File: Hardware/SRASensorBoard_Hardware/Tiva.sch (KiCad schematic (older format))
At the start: 7 parts, among them U3 TM4C129E_Launchpad

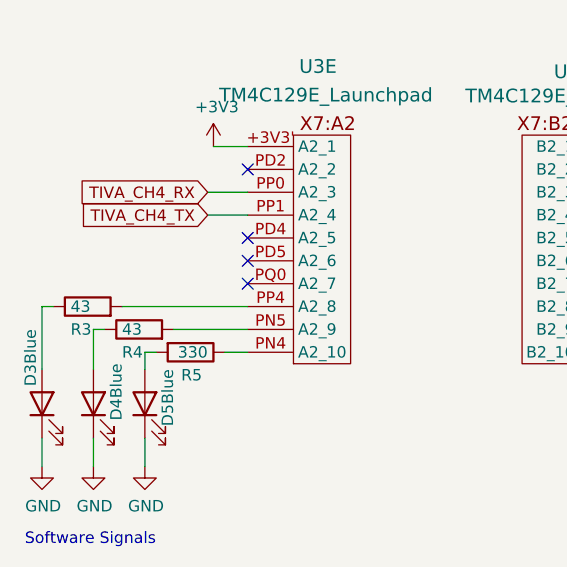
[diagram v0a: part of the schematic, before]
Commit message: rev 2 changes
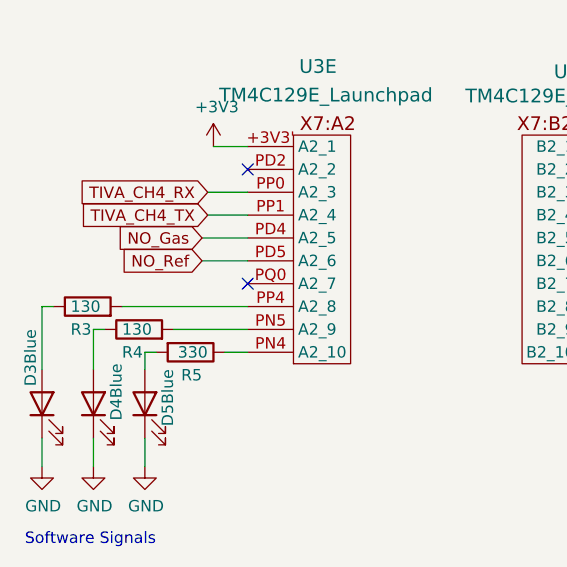
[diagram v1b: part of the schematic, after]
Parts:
- R3, R4: value 43 -> 130
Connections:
- net NO_Gas: now reaches U3.PD4 (A2_5)
- net NO_Ref: now reaches U3.PD5 (A2_6)
- no-connect marks 52 -> 50
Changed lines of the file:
@@
 Wire Wire Line
 	2000 3400 2175 3400
-Text GLabel 1850 2275 0    50   Output ~ 0
-NO2_SCL
-Text GLabel 1850 2375 0    50   Output ~ 0
-NO2_SDA
-Wire Wire Line
-	2125 2275 1850 2275
-Wire Wire Line
-	2125 2375 1850 2375
 Text GLabel 4000 3500 2    50   Input ~ 0
 TIVA_NH3_A
@@
 NoConn ~ 2125 2075
 NoConn ~ 2175 3200
-NoConn ~ 2175 3500
-NoConn ~ 2175 3600
 NoConn ~ 2175 3700
 NoConn ~ 3825 4000
@@
 NoConn ~ 6975 3825
 NoConn ~ 6975 3925
-$Comp
-L Device:LED D4
-U 1 1 6165658F
-P 1500 4225
-F 0 "D4" H 1475 4125 50  0000 C CNN
-F 1 "Blue" H 1600 4125 50  0000 C CNN
-F 2 "LED_SMD:LED_0603_1608Metric_Pad1.05x0.95mm_HandSolder" H 1500 4225 50  0001 C CNN
-F 3 "~" H 1500 4225 50  0001 C CNN
-	1    1500 4225
-	0    -1   -1   0
-$EndComp
-Wire Wire Line
-	2175 3800 1625 3800
-Wire Wire Line
-	1850 3900 2175 3900
-Wire Wire Line
-	2075 4000 2175 4000
-Wire Wire Line
-	1775 4000 1725 4000
-Wire Wire Line
-	1725 4000 1725 4075
-$Comp
-L Device:R R4
-U 1 1 6165C9F3
-P 1700 3900
-F 0 "R4" V 1600 3975 50  0000 R CNN
-F 1 "43" V 1700 3975 50  0000 R CNN
-F 2 "Resistor_SMD:R_0603_1608Metric_Pad1.05x0.95mm_HandSolder" V 1630 3900 50  0001 C CNN
-F 3 "~" H 1700 3900 50  0001 C CNN
-	1    1700 3900
-	0    -1   -1   0
-$EndComp
-$Comp
-L Device:R R3
-U 1 1 6165CD26
-P 1475 3800
-F 0 "R3" V 1375 3875 50  0000 R CNN
-F 1 "43" V 1475 3875 50  0000 R CNN
-F 2 "Resistor_SMD:R_0603_1608Metric_Pad1.05x0.95mm_HandSolder" V 1405 3800 50  0001 C CNN
-F 3 "~" H 1475 3800 50  0001 C CNN
-	1    1475 3800
-	0    -1   -1   0
-$EndComp
-$Comp
-L Device:LED D3
-U 1 1 616555A2
-P 1275 4225
-F 0 "D3" H 1400 4275 50  0000 C CNN
-F 1 "Blue" H 1525 4275 50  0000 C CNN
-F 2 "LED_SMD:LED_0603_1608Metric_Pad1.05x0.95mm_HandSolder" H 1275 4225 50  0001 C CNN
-F 3 "~" H 1275 4225 50  0001 C CNN
-	1    1275 4225
-	0    -1   -1   0
-$EndComp
-Wire Wire Line
-	1550 3900 1500 3900
-Wire Wire Line
-	1500 3900 1500 4075
-Wire Wire Line
-	1325 3800 1275 3800
-Wire Wire Line
-	1275 3800 1275 4075
-$Comp
-L power:GND #PWR0119
-U 1 1 61666E76
-P 1500 4500
-F 0 "#PWR0119" H 1500 4250 50  0001 C CNN
-F 1 "GND" H 1505 4327 50  0000 C CNN
-F 2 "" H 1500 4500 50  0001 C CNN
-F 3 "" H 1500 4500 50  0001 C CNN
-	1    1500 4500
-	1    0    0    -1
-$EndComp
-$Comp
-L power:GND #PWR0120
-U 1 1 6166AD67
-P 1725 4500
-F 0 "#PWR0120" H 1725 4250 50  0001 C CNN
-F 1 "GND" H 1730 4327 50  0000 C CNN
-F 2 "" H 1725 4500 50  0001 C CNN
-F 3 "" H 1725 4500 50  0001 C CNN
-	1    1725 4500
-	1    0    0    -1
-$EndComp
-$Comp
-L power:GND #PWR0121
-U 1 1 6166AEA5
-P 1275 4500
-F 0 "#PWR0121" H 1275 4250 50  0001 C CNN
-F 1 "GND" H 1280 4327 50  0000 C CNN
-F 2 "" H 1275 4500 50  0001 C CNN
-F 3 "" H 1275 4500 50  0001 C CNN
-	1    1275 4500
-	1    0    0    -1
-$EndComp
-Wire Wire Line
-	1275 4375 1275 4500
-Wire Wire Line
-	1500 4375 1500 4500
-Wire Wire Line
-	1725 4375 1725 4500
 Text Notes 1200 4850 0    50   ~ 0
 Software Signals
@@
 Wire Wire Line
 	3675 1875 3875 1875
+Text GLabel 1975 3500 0    50   Input ~ 0
+NO_Gas
+Text GLabel 1975 3600 0    50   Input ~ 0
+NO_Ref
+Wire Wire Line
+	2175 3500 1975 3500
+Wire Wire Line
+	2175 3600 1975 3600
+$Comp
+L Device:LED D5
+U 1 1 6165680B
+P 1725 4225
+F 0 "D5" H 1675 4125 50  0000 C CNN
+F 1 "Blue" H 1800 4125 50  0000 C CNN
+F 2 "LED_SMD:LED_0603_1608Metric_Pad1.05x0.95mm_HandSolder" H 1725 4225 50  0001 C CNN
+F 3 "~" H 1725 4225 50  0001 C CNN
+	1    1725 4225
+	0    -1   -1   0
+$EndComp
 $Comp
 L Device:R R5
@@
 	0    1    1    0
 $EndComp
-$Comp
-L Device:LED D5
-U 1 1 6165680B
-P 1725 4225
-F 0 "D5" H 1675 4125 50  0000 C CNN
-F 1 "Blue" H 1800 4125 50  0000 C CNN
-F 2 "LED_SMD:LED_0603_1608Metric_Pad1.05x0.95mm_HandSolder" H 1725 4225 50  0001 C CNN
-F 3 "~" H 1725 4225 50  0001 C CNN
-	1    1725 4225
-	0    -1   -1   0
-$EndComp
+Wire Wire Line
+	1725 4375 1725 4500
+Wire Wire Line
+	1500 4375 1500 4500
+Wire Wire Line
+	1275 4375 1275 4500
+$Comp
+L power:GND #PWR0121
+U 1 1 6166AEA5
+P 1275 4500
+F 0 "#PWR0121" H 1275 4250 50  0001 C CNN
+F 1 "GND" H 1280 4327 50  0000 C CNN
+F 2 "" H 1275 4500 50  0001 C CNN
+F 3 "" H 1275 4500 50  0001 C CNN
+	1    1275 4500
+	1    0    0    -1
+$EndComp
+$Comp
+L power:GND #PWR0120
+U 1 1 6166AD67
+P 1725 4500
+F 0 "#PWR0120" H 1725 4250 50  0001 C CNN
+F 1 "GND" H 1730 4327 50  0000 C CNN
+F 2 "" H 1725 4500 50  0001 C CNN
+F 3 "" H 1725 4500 50  0001 C CNN
+	1    1725 4500
+	1    0    0    -1
+$EndComp
+$Comp
+L power:GND #PWR0119
+U 1 1 61666E76
+P 1500 4500
+F 0 "#PWR0119" H 1500 4250 50  0001 C CNN
+F 1 "GND" H 1505 4327 50  0000 C CNN
+F 2 "" H 1500 4500 50  0001 C CNN
+F 3 "" H 1500 4500 50  0001 C CNN
+	1    1500 4500
+	1    0    0    -1
+$EndComp
+Wire Wire Line
+	1275 3800 1275 4075
+Wire Wire Line
+	1325 3800 1275 3800
+Wire Wire Line
+	1500 3900 1500 4075
+Wire Wire Line
+	1550 3900 1500 3900
+$Comp
+L Device:LED D3
+U 1 1 616555A2
+P 1275 4225
+F 0 "D3" H 1400 4275 50  0000 C CNN
+F 1 "Blue" H 1525 4275 50  0000 C CNN
+F 2 "LED_SMD:LED_0603_1608Metric_Pad1.05x0.95mm_HandSolder" H 1275 4225 50  0001 C CNN
+F 3 "~" H 1275 4225 50  0001 C CNN
+	1    1275 4225
+	0    -1   -1   0
+$EndComp
+$Comp
+L Device:R R3
+U 1 1 6165CD26
+P 1475 3800
+F 0 "R3" V 1375 3875 50  0000 R CNN
+F 1 "130" V 1475 3875 50  0000 R CNN
+F 2 "Resistor_SMD:R_0603_1608Metric_Pad1.05x0.95mm_HandSolder" V 1405 3800 50  0001 C CNN
+F 3 "~" H 1475 3800 50  0001 C CNN
+	1    1475 3800
+	0    -1   -1   0
+$EndComp
+Wire Wire Line
+	1725 4000 1725 4075
+Wire Wire Line
+	1775 4000 1725 4000
+Wire Wire Line
+	2075 4000 2175 4000
+Wire Wire Line
+	1850 3900 2175 3900
+Wire Wire Line
+	2175 3800 1625 3800
+$Comp
+L Device:LED D4
+U 1 1 6165658F
+P 1500 4225
+F 0 "D4" H 1475 4125 50  0000 C CNN
+F 1 "Blue" H 1600 4125 50  0000 C CNN
+F 2 "LED_SMD:LED_0603_1608Metric_Pad1.05x0.95mm_HandSolder" H 1500 4225 50  0001 C CNN
+F 3 "~" H 1500 4225 50  0001 C CNN
+	1    1500 4225
+	0    -1   -1   0
+$EndComp
+Text GLabel 1850 2275 0    50   Output ~ 0
+NO2_SCL
+Text GLabel 1850 2375 0    50   Output ~ 0
+NO2_SDA
+Wire Wire Line
+	2125 2275 1850 2275
+Wire Wire Line
+	2125 2375 1850 2375
+$Comp
+L Device:R R4
+U 1 1 6165C9F3
+P 1700 3900
+F 0 "R4" V 1600 3975 50  0000 R CNN
+F 1 "130" V 1700 3975 50  0000 R CNN
+F 2 "Resistor_SMD:R_0603_1608Metric_Pad1.05x0.95mm_HandSolder" V 1630 3900 50  0001 C CNN
+F 3 "~" H 1700 3900 50  0001 C CNN
+	1    1700 3900
+	0    -1   -1   0
+$EndComp
